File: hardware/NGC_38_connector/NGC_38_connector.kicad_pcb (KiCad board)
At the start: 2 copper layers, 38 x 29 mm, 5 parts, among them P1 DIL38, P2 CONN_10, P3 CONN_9, P4 CONN_10, P5 CONN_9

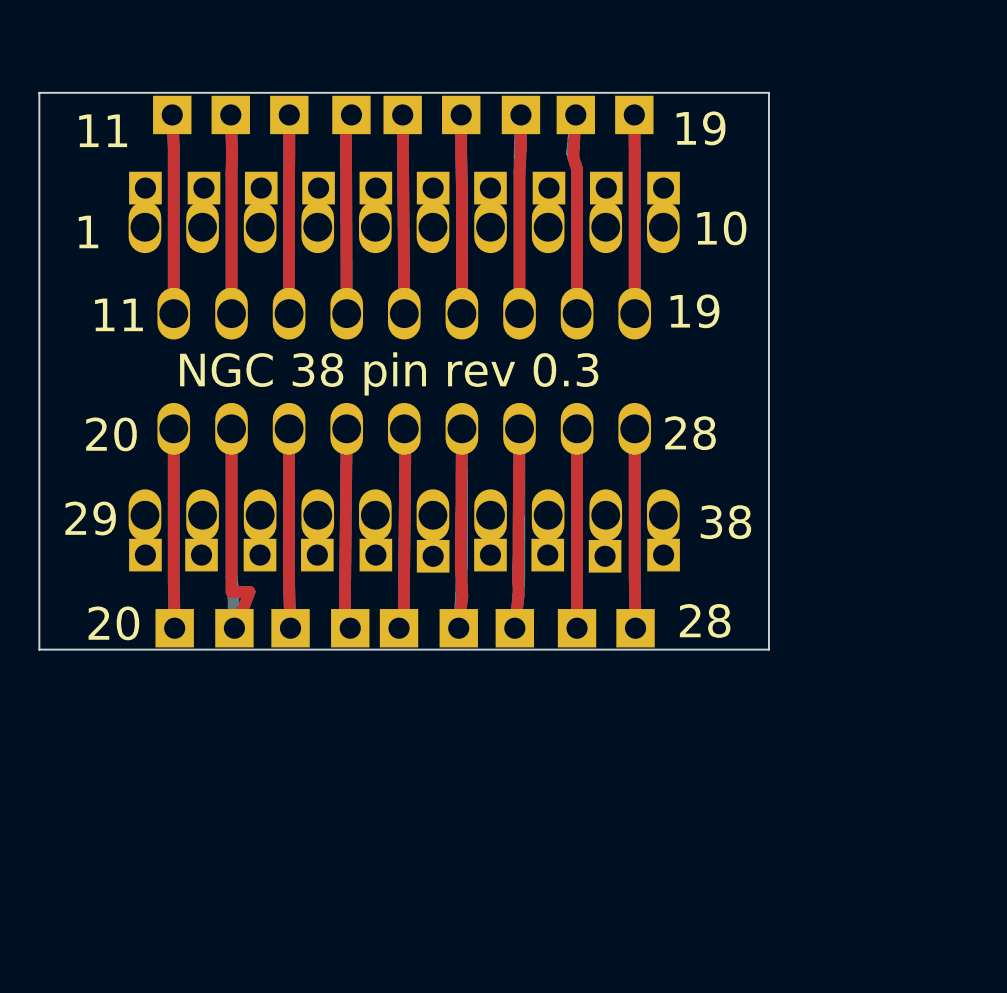
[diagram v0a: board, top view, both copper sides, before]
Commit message: auto-sync
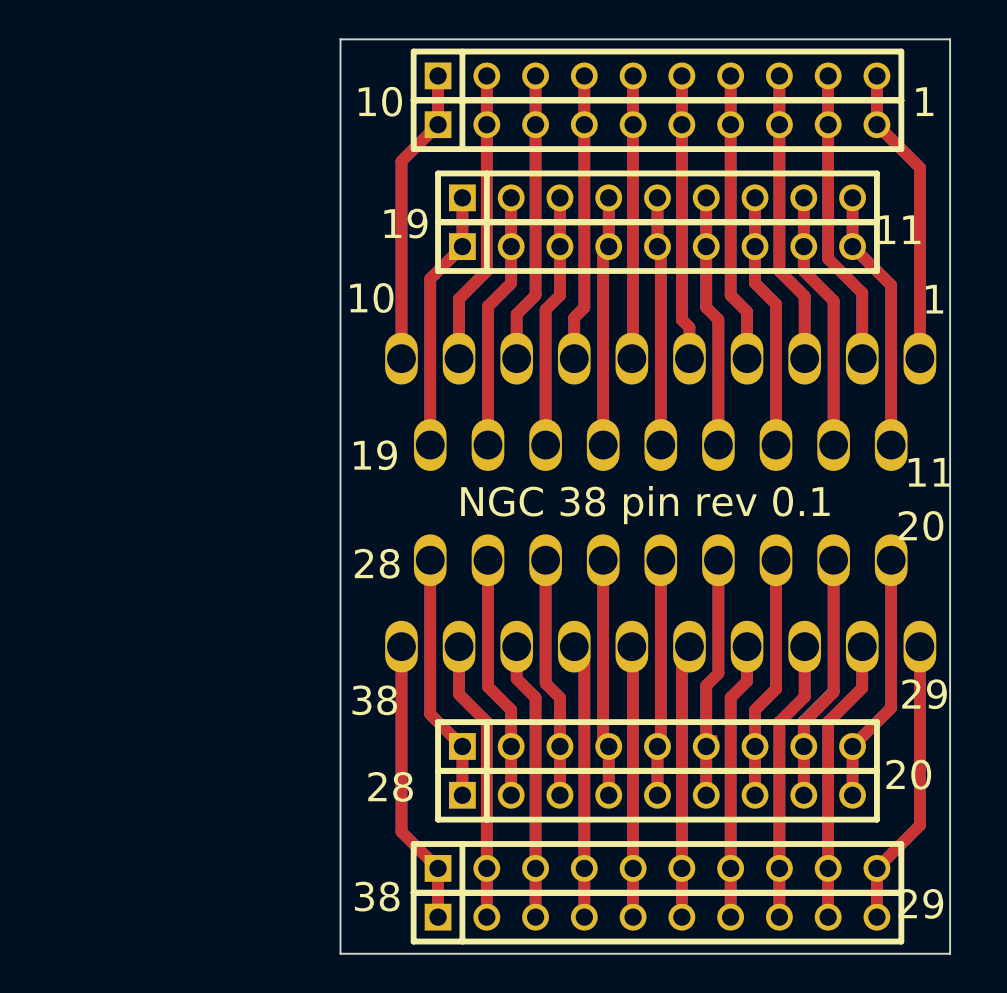
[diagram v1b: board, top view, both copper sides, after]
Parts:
- added P6: CONN_10, SIL-10, F.Cu at (163.2, 134.6)
- added P7: CONN_9, SIL-9, F.Cu at (163.2, 141.0)
- added P8: CONN_9, SIL-9, F.Cu at (163.2, 172.1)
- added P9: CONN_10, SIL-10, F.Cu at (163.2, 178.4)
- moved P4 21.4 mm to (163.2, 175.9)
- moved P3 15.1 mm to (163.2, 143.5)
- moved P1 15.0 mm to (149.9, 156.8)
- moved P5 14.8 mm to (163.2, 169.5)
- moved P2 13.9 mm to (163.2, 137.2)
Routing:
- net N-0000010: track 2.04 -> 31.3 mm
- net N-000001: track 2.05 -> 31.0 mm
- net N-000009: track 2.05 -> 30.9 mm
- net N-000002: track 2.07 -> 30.6 mm
- net N-000008: track 2.06 -> 30.5 mm
- net N-000003: track 2.06 -> 30.3 mm
- net N-000007: track 2.04 -> 30.2 mm
- net N-0000035: track 2.08 -> 30.0 mm
- net N-000004: track 2.06 -> 29.9 mm
- net N-000006: track 2.04 -> 29.8 mm
- net N-0000027: track 2.09 -> 29.8 mm
- net N-0000034: track 2.15 -> 29.7 mm
- net N-000005: track 2.05 -> 29.5 mm
- net N-0000028: track 2.10 -> 29.4 mm
- net N-0000033: track 2.08 -> 29.3 mm
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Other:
- board size 38 x 29 mm -> 31.8 x 47.6 mm
- board text added: "NGC 38 pin rev 0.1"
- board text removed: "NGC 38 pin rev 0.3"

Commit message: auto-sync
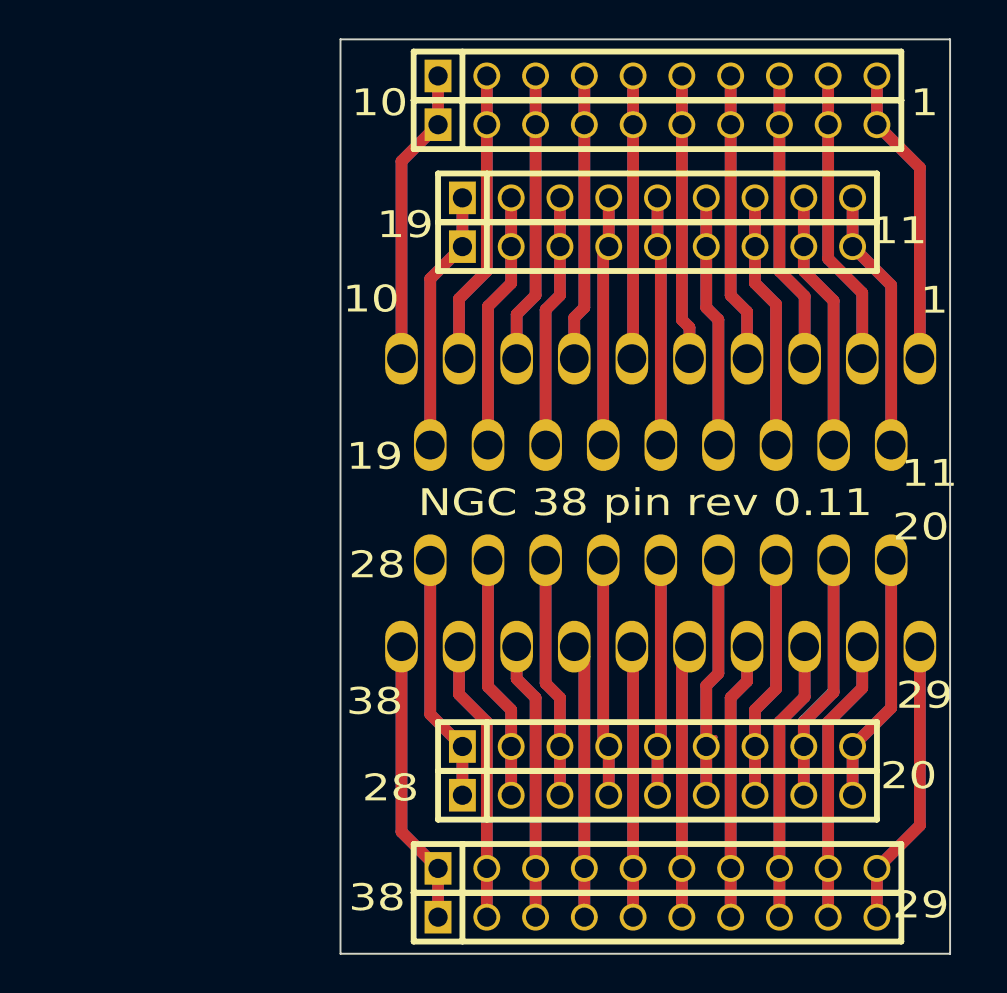
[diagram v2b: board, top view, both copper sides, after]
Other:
- board text added: "NGC 38 pin rev 0.11"
- board text removed: "NGC 38 pin rev 0.1"

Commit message: auto-sync
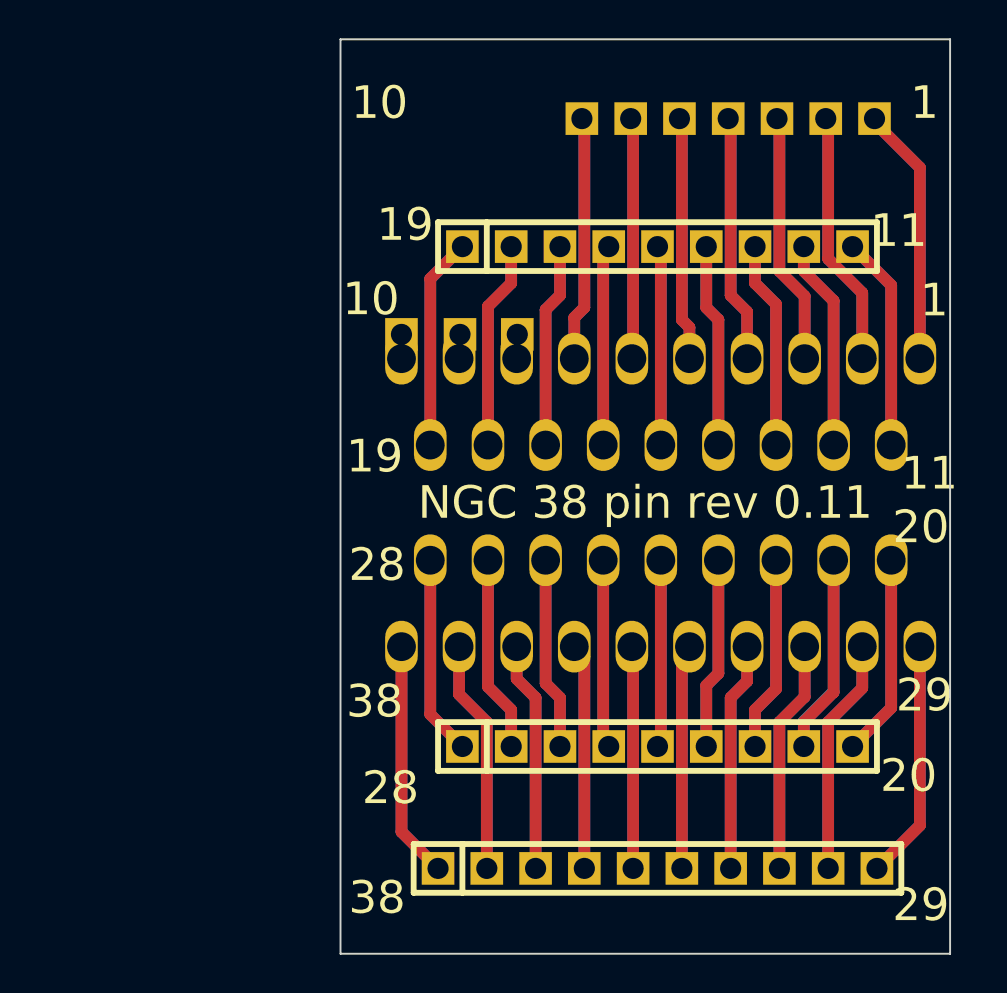
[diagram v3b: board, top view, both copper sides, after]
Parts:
- removed P6, P9: CONN_10, SIL-10
- removed P7, P8: CONN_9, SIL-9
- moved P2 0.34 mm to (163.1, 136.8)
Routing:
- net N-0000011: track 31.0 -> 0.00 mm
- net N-0000010: track 30.6 -> 0.00 mm
- net N-000009: track 30.3 -> 0.00 mm
- net N-0000028: track 25.5 -> 20.4 mm
- net N-0000027: track 25.1 -> 20.0 mm
- net N-0000026: track 25.3 -> 20.3 mm
- net N-0000025: track 24.6 -> 19.6 mm
- net N-0000024: track 25.7 -> 20.6 mm
- net N-0000023: track 25.4 -> 20.3 mm
- net N-0000022: track 25.8 -> 20.7 mm
- net N-0000021: track 26.1 -> 21.1 mm
- net N-0000016: track 25.9 -> 20.8 mm
- net N-000008: track 29.9 -> 24.8 mm
- net N-000007: track 29.5 -> 24.4 mm
- net N-000006: track 29.8 -> 24.7 mm
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
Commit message: auto-sync
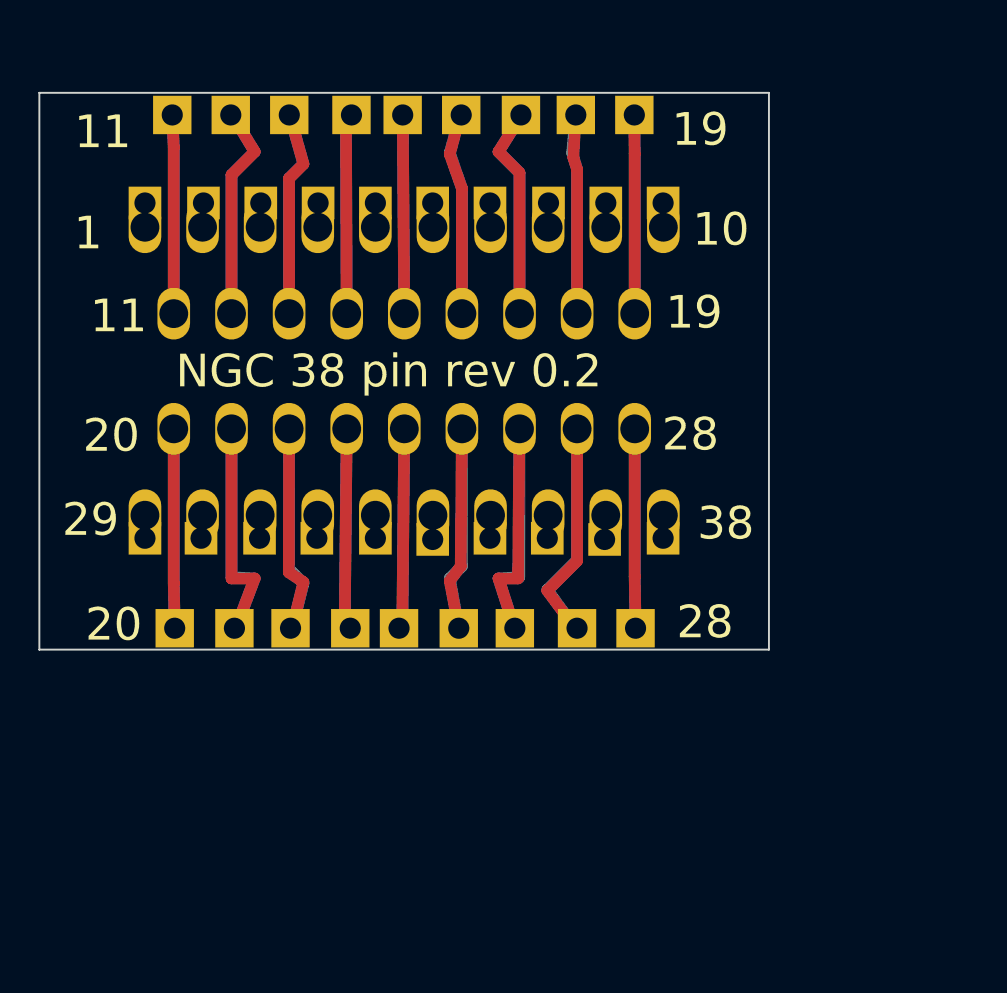
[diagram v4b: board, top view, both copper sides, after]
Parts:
- moved P4 22.1 mm to (149.3, 158.7)
- moved P3 15.1 mm to (149.8, 136.7)
- moved P1 15.0 mm to (136.5, 150.0)
- moved P5 14.8 mm to (149.7, 163.4)
- moved P2 14.1 mm to (149.7, 141.2)
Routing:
- net N-000002: track 26.2 -> 0.00 mm
- net N-000003: track 25.8 -> 0.00 mm
- net N-000004: track 25.5 -> 0.00 mm
- net N-000005: track 25.1 -> 0.00 mm
- net N-0000033: track 25.0 -> 0.00 mm
- net N-000008: track 24.8 -> 0.00 mm
- net N-000006: track 24.7 -> 0.00 mm
- net N-0000035: track 24.7 -> 0.00 mm
- net N-0000036: track 24.6 -> 0.00 mm
- net N-000007: track 24.4 -> 0.00 mm
- net N-0000034: track 24.3 -> 0.00 mm
- net N-0000037: track 24.2 -> 0.00 mm
- net N-0000029: track 23.9 -> 0.00 mm
- net N-0000038: track 23.8 -> 0.00 mm
- net N-0000032: track 23.5 -> 0.00 mm
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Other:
- board size 31.8 x 47.6 mm -> 38 x 29 mm
- board text added: "NGC 38 pin rev 0.2"
- board text removed: "NGC 38 pin rev 0.11"
